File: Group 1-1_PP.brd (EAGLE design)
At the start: 90 x 75 mm, 40 parts, among them IC1 74LS90N, IC10 7805T, IC2 74LS90N, IC3 74LS48N, IC4 74LS48N, IC5 74ALS08N, IC6 LM555N, IC7 74LS14N, IC8 7476N, IC9 74LS32N

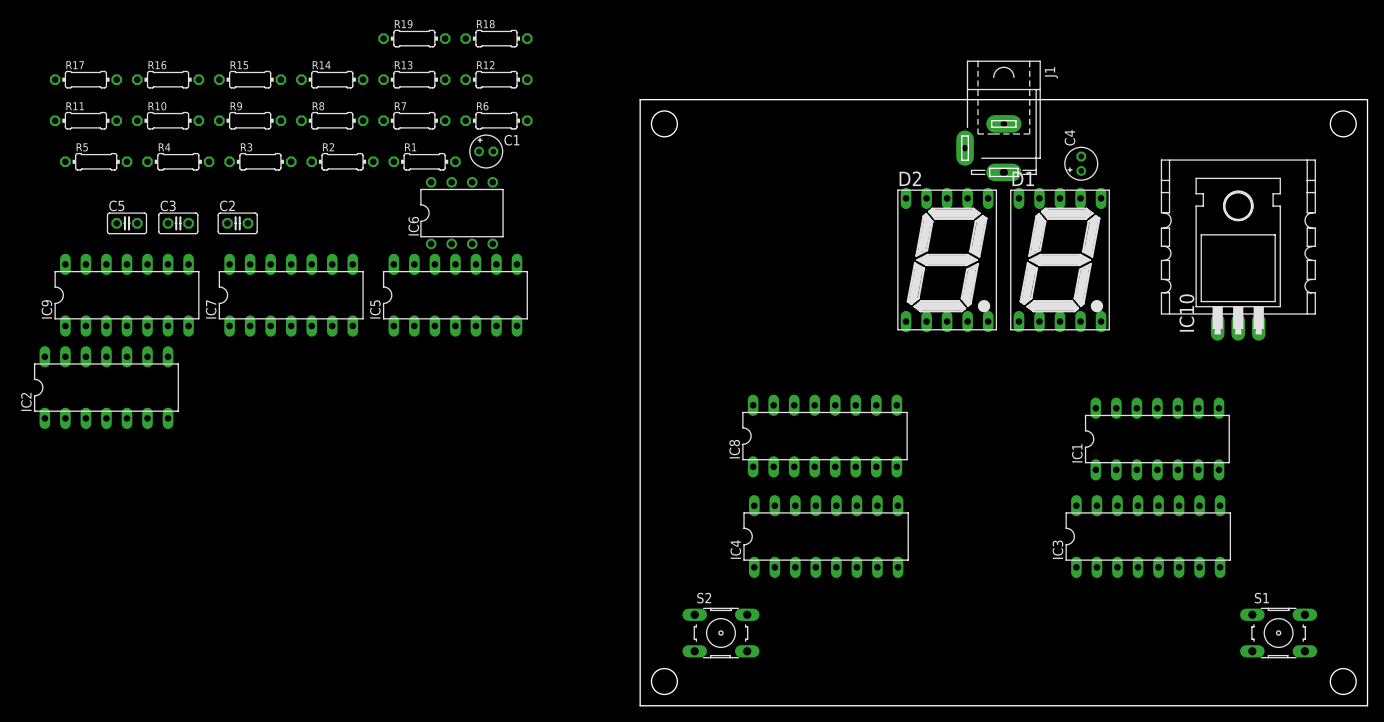
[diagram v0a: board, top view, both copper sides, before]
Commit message: MANAAAAAAAAAAAAAAAAAAAA
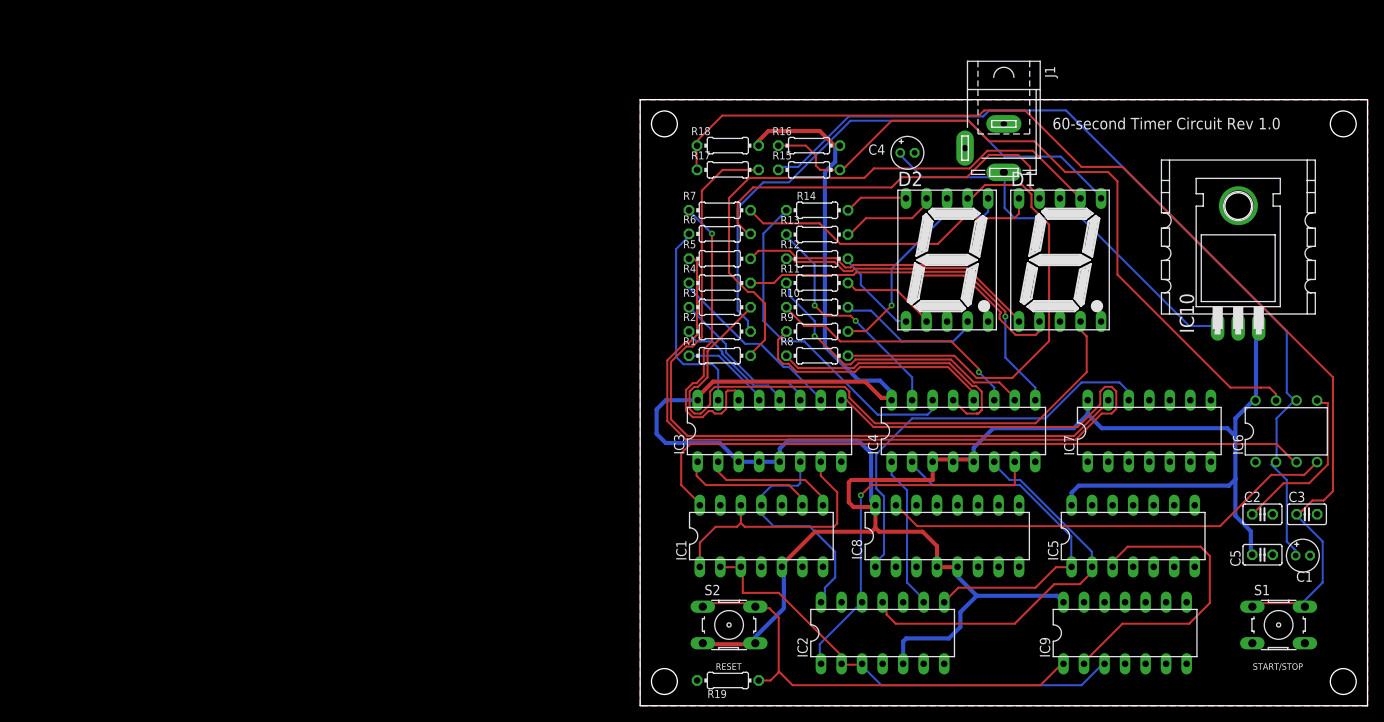
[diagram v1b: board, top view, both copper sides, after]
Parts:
- moved C5 146.4 mm to (77.0, 18.7)
- moved C3 144.2 mm to (82.5, 23.7)
- moved C2 131.8 mm to (77.0, 23.7)
- moved IC9 130.4 mm to (60.0, 9.00)
- moved C1 112.7 mm to (82.0, 18.6)
- moved IC7 107.5 mm to (63.0, 34.0)
- moved IC6 105.5 mm to (80.0, 34.0)
- moved IC2 100.7 mm to (30.0, 9.00)
- moved R11 92.7 mm to (21.9, 52.3)
- moved IC5 89.0 mm to (61.0, 21.0)
- moved R19 88.4 mm to (10.9, 3.13)
- moved R10 83.6 mm to (21.9, 49.3)
- moved R17 80.2 mm to (10.8, 66.3)
- moved R16 79.7 mm to (20.9, 69.3)
- moved R5 78.1 mm to (9.85, 55.3)
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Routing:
- net VCC: track 0.00 -> 316.4 mm
- net N$4: track 0.00 -> 138.4 mm
- net N$14: track 0.00 -> 121.5 mm
- net TR: track 0.00 -> 108.5 mm
- net N$3: track 0.00 -> 96.2 mm
- net N$7: track 0.00 -> 87.6 mm
- net CLK_1HZ: track 0.00 -> 84.8 mm
- net N$21: track 0.00 -> 79.5 mm
- net N$23: track 0.00 -> 70.8 mm
- net N$22: track 0.00 -> 69.7 mm
- net RESET: track 0.00 -> 57.9 mm
- net N$5: track 0.00 -> 57.0 mm
- net STRST: track 0.00 -> 56.5 mm
- net N$30: track 0.00 -> 56.0 mm
- net N$1: track 0.00 -> 51.3 mm
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- added copper zone on layer 1, net GND
- added copper zone on layer 16, net GND
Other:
- board text added: "60-second Timer Circuit Rev 1.0"
- board text added: "RESET"
- board text added: "START/STOP"
